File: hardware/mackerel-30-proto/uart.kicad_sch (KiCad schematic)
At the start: 6 parts, among them U5 XR68C681, X2 3.6864MHz

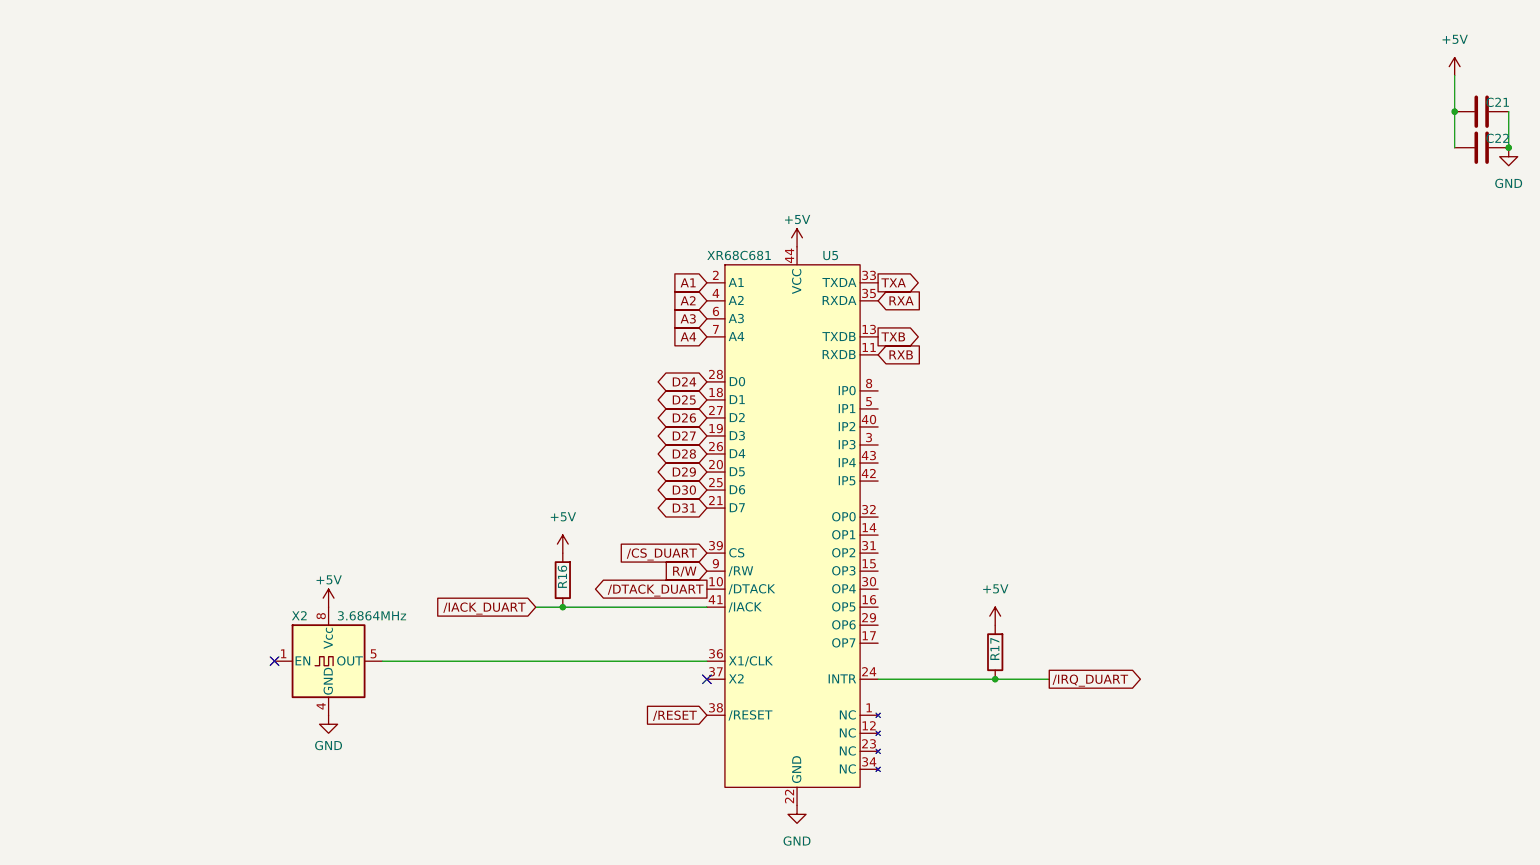
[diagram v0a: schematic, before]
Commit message: positioning
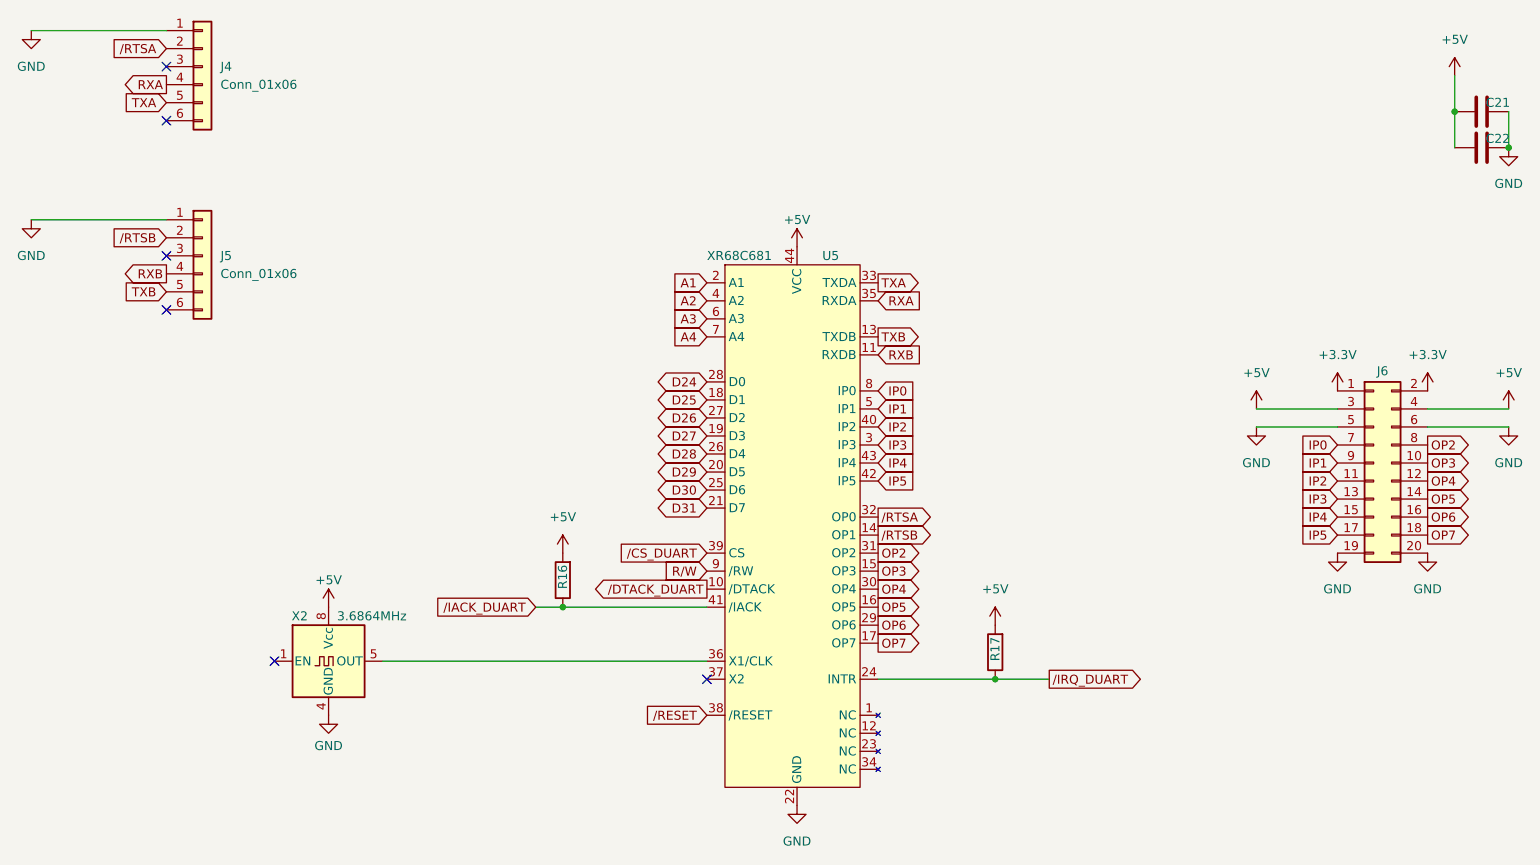
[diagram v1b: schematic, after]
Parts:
- added J4, J5: Conn_01x06, Connector_PinHeader_2.54mm:PinHeader_1x06_P2.54mm_Vertical, symbol Connector_Generic:Conn_01x06
- added J6: Conn_02x10_Odd_Even, Connector_PinHeader_2.54mm:PinHeader_2x10_P2.54mm_Vertical, symbol Connector_Generic:Conn_02x10_Odd_Even
- C21, C22: footprint Capacitor_SMD:C_1210_3225Metric_Pad1.33x2.70mm_HandSolder -> Capacitor_SMD:C_1206_3216Metric_Pad1.33x1.80mm_HandSolder
- R16, R17: footprint Resistor_THT:R_Axial_DIN0207_L6.3mm_D2.5mm_P7.62mm_Horizontal -> Resistor_SMD:R_0805_2012Metric_Pad1.20x1.40mm_HandSolder
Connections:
- net +5V: now also J6.3 (Pin_3), J6.4 (Pin_4)
- net GND: now also J4.1 (Pin_1), J5.1 (Pin_1), J6.19 (Pin_19), J6.20 (Pin_20), J6.5 (Pin_5), J6.6 (Pin_6)
- net RXA: now also J4.4 (Pin_4)
- net RXB: now also J5.4 (Pin_4)
- net TXA: now also J4.5 (Pin_5)
- net TXB: now also J5.5 (Pin_5)
- net /RTSB: now reaches U5.14 (OP1)
- net /RTSB: now also J5.2 (Pin_2)
- net OP3: now reaches U5.15 (OP3)
- net OP3: now also J6.10 (Pin_10)
- net OP5: now reaches U5.16 (OP5)
- net OP5: now also J6.14 (Pin_14)
- net OP7: now reaches U5.17 (OP7)
- net OP7: now also J6.18 (Pin_18)
- net OP6: now reaches U5.29 (OP6)
- net OP6: now also J6.16 (Pin_16)
- net IP3: now reaches U5.3 (IP3)
- net IP3: now also J6.13 (Pin_13)
- net OP4: now reaches U5.30 (OP4)
- net OP4: now also J6.12 (Pin_12)
- net OP2: now reaches U5.31 (OP2)
- net OP2: now also J6.8 (Pin_8)
- net /RTSA: now reaches U5.32 (OP0)
- net /RTSA: now also J4.2 (Pin_2)
- net IP2: now reaches U5.40 (IP2)
- net IP2: now also J6.11 (Pin_11)
- net IP5: now reaches U5.42 (IP5)
- net IP5: now also J6.17 (Pin_17)
- net IP4: now reaches U5.43 (IP4)
- net IP4: now also J6.15 (Pin_15)
- net IP1: now reaches U5.5 (IP1)
- net IP1: now also J6.9 (Pin_9)
- net IP0: now reaches U5.8 (IP0)
- net IP0: now also J6.7 (Pin_7)
- new net +3.3V: J6.1 (Pin_1), J6.2 (Pin_2)
- no-connect marks 2 -> 6
